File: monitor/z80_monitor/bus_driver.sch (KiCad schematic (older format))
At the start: 15 parts, among them J1 Conn_02x25_Odd_Even, U1 74HC237, U10 74HCT365, U11 74HC573, U12 74LS05, U2 74HCT245, U3 74HC573, U4 74LS04, U5 74HC32, U6 74LS00, U7 74HC573, U8 74HC573, U9 74HCT365

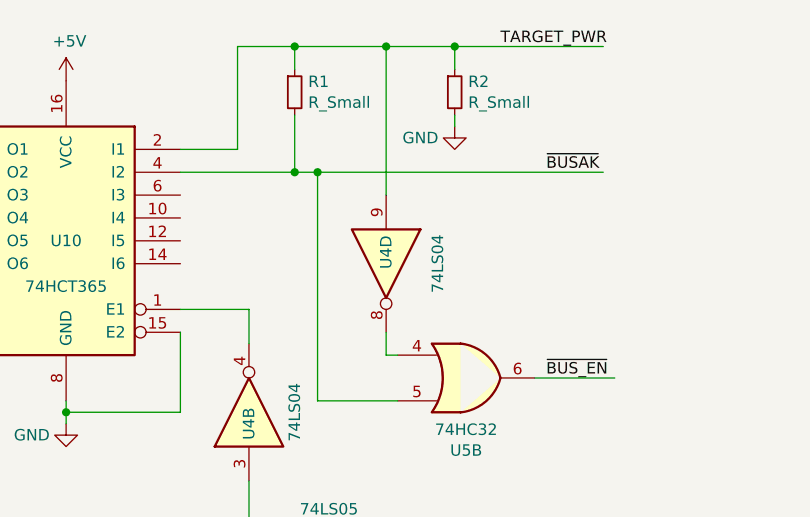
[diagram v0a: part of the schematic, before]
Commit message: More updates.
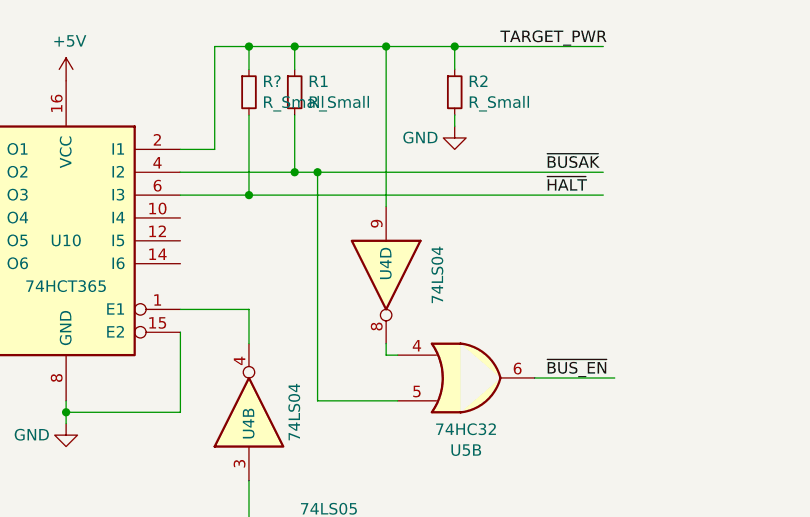
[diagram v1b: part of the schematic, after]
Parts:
- added R?: R_Small, Resistors_ThroughHole:R_Axial_DIN0411_L9.9mm_D3.6mm_P12.70mm_Horizontal, symbol Device:R_Small
- U11, U3, U7, U8: footprint Housings_DIP:DIP-20_W7.62mm... -> Housings_DIP:DIP-20_W7.62mm
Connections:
- wire segments 269 -> 274
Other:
- moved on the sheet: U4D
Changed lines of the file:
@@
 F 0 "U7" H 3950 3950 50  0000 C CNN
 F 1 "74HC573" H 3950 3600 50  0000 C CNN
-F 2 "Housings_DIP:DIP-20_W7.62mm..." H 3950 3900 50  0001 C CNN
+F 2 "Housings_DIP:DIP-20_W7.62mm" H 3950 3900 50  0001 C CNN
 F 3 "" H 3950 3900 50  0001 C CNN
 	1    3950 3900
@@
 F 0 "U11" H 7500 3950 50  0000 C CNN
 F 1 "74HC573" H 7500 3600 50  0000 C CNN
-F 2 "Housings_DIP:DIP-20_W7.62mm..." H 7500 3900 50  0001 C CNN
+F 2 "Housings_DIP:DIP-20_W7.62mm" H 7500 3900 50  0001 C CNN
 F 3 "" H 7500 3900 50  0001 C CNN
 	1    7500 3900
@@
 F 0 "U8" H 5750 3950 50  0000 C CNN
 F 1 "74HC573" H 5750 3600 50  0000 C CNN
-F 2 "Housings_DIP:DIP-20_W7.62mm..." H 5750 3900 50  0001 C CNN
+F 2 "Housings_DIP:DIP-20_W7.62mm" H 5750 3900 50  0001 C CNN
 F 3 "" H 5750 3900 50  0001 C CNN
 	1    5750 3900
@@
 F 0 "U3" H 2200 3950 50  0000 C CNN
 F 1 "74HC573" H 2200 3600 50  0000 C CNN
-F 2 "Housings_DIP:DIP-20_W7.62mm..." H 2200 3900 50  0001 C CNN
+F 2 "Housings_DIP:DIP-20_W7.62mm" H 2200 3900 50  0001 C CNN
 F 3 "" H 2200 3900 50  0001 C CNN
 	1    2200 3900
@@
 ~BUS_EN~
 Wire Wire Line
-	8000 1150 8250 1150
+	8000 1150 8150 1150
 Wire Wire Line
 	8000 1250 8500 1250
-$Comp
-L 74xx:74LS04 U4
-U 4 1 5FE8F245
-P 8900 1650
-F 0 "U4" H 8850 1650 50  0000 C CNN
-F 1 "74LS04" H 8900 1876 50  0000 C CNN
-F 2 "Housings_DIP:DIP-14_W7.62mm" H 8900 1650 50  0001 C CNN
-F 3 "" H 8900 1650 50  0001 C CNN
-	4    8900 1650
-	0    1    1    0
-$EndComp
 $Comp
 L Device:R_Small R2
@@
 $EndComp
 Wire Wire Line
-	8250 700  8500 700
+	8150 700  8300 700
 $Comp
 L Device:R_Small R1
@@
 	8500 1250 8600 1250
 Wire Wire Line
-	8900 1350 8900 700
+	8900 1400 8900 700
 Connection ~ 8900 700
 Wire Wire Line
 	8900 700  9200 700
 Wire Wire Line
-	8250 700  8250 1150
+	8150 700  8150 1150
 Wire Wire Line
 	9200 800  9200 700
@@
 Wire Wire Line
 	8950 2050 8900 2050
-Wire Wire Line
-	8900 2050 8900 1950
 Wire Wire Line
 	8950 2250 8600 2250
@@
 Wire Wire Line
 	8400 3900 8500 3900
+Wire Wire Line
+	8900 2050 8900 2000
+$Comp
+L 74xx:74LS04 U4
+U 4 1 5FE8F245
+P 8900 1700
+F 0 "U4" H 8850 1700 50  0000 C CNN
+F 1 "74LS04" H 8900 1926 50  0000 C CNN
+F 2 "Housings_DIP:DIP-14_W7.62mm" H 8900 1700 50  0001 C CNN
+F 3 "" H 8900 1700 50  0001 C CNN
+	4    8900 1700
+	0    1    1    0
+$EndComp
+Wire Wire Line
+	8000 1350 8300 1350
+Text Label 9600 1350 0    50   ~ 0
+~HALT~
+$Comp
+L Device:R_Small R?
+U 1 1 5FD3F7AE
+P 8300 900
+F 0 "R?" H 8359 946 50  0000 L CNN
+F 1 "R_Small" H 8359 855 50  0000 L CNN
+F 2 "Resistors_ThroughHole:R_Axial_DIN0411_L9.9mm_D3.6mm_P12.70mm_Horizontal" H 8300 900 50  0001 C CNN
+F 3 "~" H 8300 900 50  0001 C CNN
+	1    8300 900
+	1    0    0    -1
+$EndComp
+Wire Wire Line
+	8300 1000 8300 1350
+Connection ~ 8300 1350
+Wire Wire Line
+	8300 1350 9850 1350
+Wire Wire Line
+	8300 800  8300 700
 Wire Bus Line
 	1100 5150 6650 5150
@@
 Wire Bus Line
 	1450 1200 1450 5050
+Connection ~ 8300 700
+Wire Wire Line
+	8300 700  8500 700
 $EndSCHEMATC
